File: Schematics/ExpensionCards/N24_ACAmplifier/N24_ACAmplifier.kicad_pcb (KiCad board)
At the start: 2 copper layers, 97 x 76 mm, 14 parts

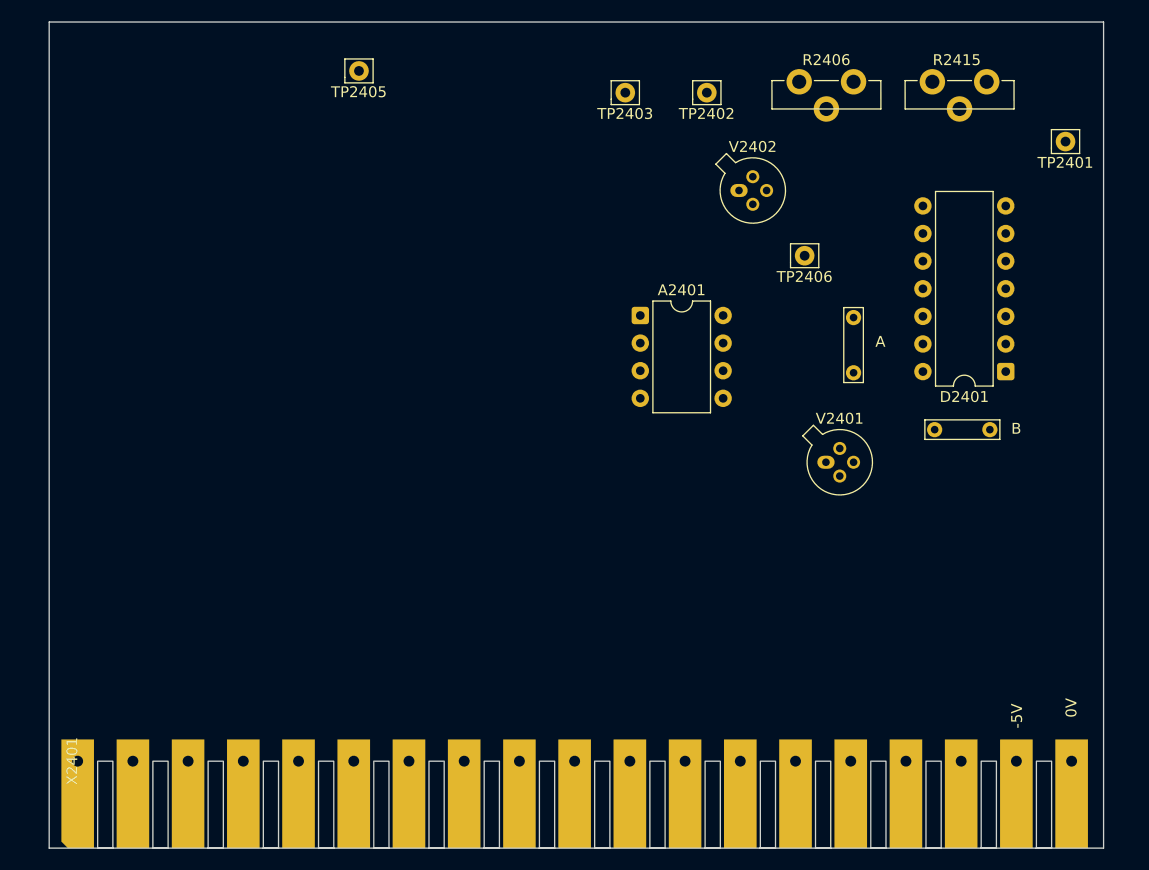
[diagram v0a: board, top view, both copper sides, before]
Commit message: Updated N24 schema/PCB
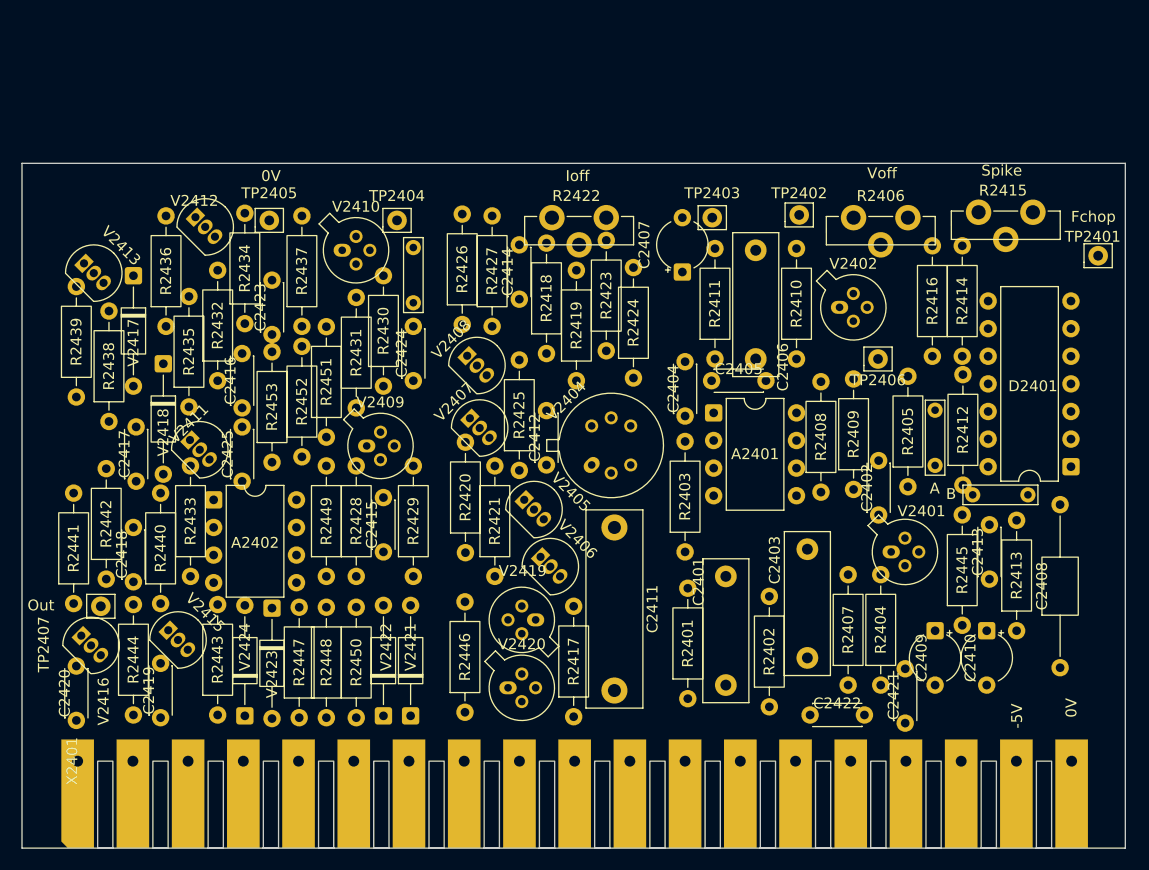
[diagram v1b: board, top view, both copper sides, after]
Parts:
- added A2402: LM393N, Package_DIP:DIP-8_W7.62mm, F.Cu at (114.1, 122.5)
- added C2401: 22n, Capacitor_THT:C_Rect_L13.0mm_W4.0mm_P10.00mm_FKS3_FKP3_MKS4, F.Cu at (161.2, 139.5)
- added C2402: 8p2, Capacitor_THT:C_Disc_D4.3mm_W1.9mm_P5.00mm, F.Cu at (175.3, 123.8)
- added C2403: 33n, Capacitor_THT:C_Rect_L13.0mm_W4.0mm_P10.00mm_FKS3_FKP3_MKS4, F.Cu at (168.8, 137.0)
- added C2404: 220p, Capacitor_THT:C_Disc_D4.3mm_W1.9mm_P5.00mm, F.Cu at (157.5, 114.8)
- added C2405: 3p9, Capacitor_THT:C_Disc_D4.3mm_W1.9mm_P5.00mm, F.Cu at (159.9, 111.5)
- added C2406: 220n, Capacitor_THT:C_Rect_L13.0mm_W4.0mm_P10.00mm_FKS3_FKP3_MKS4, F.Cu at (164.0, 109.5)
- added C2407: 22u, Capacitor_THT:CP_Radial_Tantal_D4.5mm_P5.00mm, F.Cu at (157.2, 101.5)
- added C2408: 13n3, Capacitor_THT:C_Axial_L5.1mm_D3.1mm_P15.00mm_Horizontal, F.Cu at (192.0, 137.9)
- added C2409: 6u8, Capacitor_THT:CP_Radial_Tantal_D4.5mm_P5.00mm, F.Cu at (180.5, 134.5)
- added C2410: 6u8, Capacitor_THT:CP_Radial_Tantal_D4.5mm_P5.00mm, F.Cu at (185.2, 134.5)
- added C2411: 330n, Capacitor_THT:C_Rect_L18.0mm_W5.0mm_P15.00mm_FKS3_FKP3, F.Cu at (151.0, 125.0)
- added C2412: 150p, Capacitor_THT:C_Disc_D4.3mm_W1.9mm_P5.00mm, F.Cu at (144.8, 119.2)
- added C2413: 10n, Capacitor_THT:C_Disc_D4.3mm_W1.9mm_P5.00mm, F.Cu at (185.5, 129.8)
- added C2414: 1n8, Capacitor_THT:C_Disc_D4.3mm_W1.9mm_P5.00mm, F.Cu at (142.2, 104.0)
- added C2415: 15p, Capacitor_THT:C_Disc_D4.3mm_W1.9mm_P5.00mm, F.Cu at (129.8, 127.2)
- added C2416: 12p, Capacitor_THT:C_Disc_D4.3mm_W1.9mm_P5.00mm, F.Cu at (116.8, 114.0)
- added C2417: 10n, Capacitor_THT:C_Disc_D4.3mm_W1.9mm_P5.00mm, F.Cu at (107.0, 120.8)
- added C2418: 560p, Capacitor_THT:C_Disc_D4.3mm_W1.9mm_P5.00mm, F.Cu at (106.8, 130.0)
- added C2419: 6n8, Capacitor_THT:C_Disc_D4.3mm_W1.9mm_P5.00mm, F.Cu at (109.2, 142.5)
- added C2420: 6n8, Capacitor_THT:C_Disc_D4.3mm_W1.9mm_P5.00mm, F.Cu at (101.5, 142.8)
- added C2421: 22n, Capacitor_THT:C_Disc_D4.3mm_W1.9mm_P5.00mm, F.Cu at (177.8, 143.0)
- added C2422: 22n, Capacitor_THT:C_Disc_D4.3mm_W1.9mm_P5.00mm, F.Cu at (169.0, 142.2)
- added C2423: 22n, Capacitor_THT:C_Disc_D4.3mm_W1.9mm_P5.00mm, F.Cu at (119.5, 107.2)
- added C2424: 22n, Capacitor_THT:C_Disc_D4.3mm_W1.9mm_P5.00mm, F.Cu at (132.5, 111.5)
- added C2425: 39p, Capacitor_THT:C_Disc_D4.3mm_W1.9mm_P5.00mm, F.Cu at (116.8, 120.8)
- added JP1: Jumper_2_Small_Bridged, TestPoint:TestPoint_Bridge_Pitch5.08mm_Drill0.7mm, F.Cu at (132.5, 104.3)
- added R2401: 1M00, Resistor_THT:R_Axial_DIN0207_L6.3mm_D2.5mm_P10.16mm_Horizontal, F.Cu at (157.8, 140.8)
- added R2402: 95k3, Resistor_THT:R_Axial_DIN0207_L6.3mm_D2.5mm_P10.16mm_Horizontal, F.Cu at (165.2, 141.5)
- added R2403: 9k53, Resistor_THT:R_Axial_DIN0207_L6.3mm_D2.5mm_P10.16mm_Horizontal, F.Cu at (157.5, 127.2)
- added R2404: 15E4, Resistor_THT:R_Axial_DIN0207_L6.3mm_D2.5mm_P10.16mm_Horizontal, F.Cu at (175.5, 139.5)
- added R2405: 681k, Resistor_THT:R_Axial_DIN0207_L6.3mm_D2.5mm_P10.16mm_Horizontal, F.Cu at (178.0, 121.2)
- added R2407: 1M00, Resistor_THT:R_Axial_DIN0207_L6.3mm_D2.5mm_P10.16mm_Horizontal, F.Cu at (172.5, 139.5)
- added R2408: 681k, Resistor_THT:R_Axial_DIN0207_L6.3mm_D2.5mm_P10.16mm_Horizontal, F.Cu at (170.0, 121.8)
- added R2409: 2k74, Resistor_THT:R_Axial_DIN0207_L6.3mm_D2.5mm_P10.16mm_Horizontal, F.Cu at (173.0, 121.5)
- added R2410: 15k4, Resistor_THT:R_Axial_DIN0207_L6.3mm_D2.5mm_P10.16mm_Horizontal, F.Cu at (167.8, 109.5)
- added R2411: 1M00, Resistor_THT:R_Axial_DIN0207_L6.3mm_D2.5mm_P10.16mm_Horizontal, F.Cu at (160.2, 109.5)
- added R2412: 1k05, Resistor_THT:R_Axial_DIN0207_L6.3mm_D2.5mm_P10.16mm_Horizontal, F.Cu at (183.1, 121.1)
- added R2413: 634k, Resistor_THT:R_Axial_DIN0207_L6.3mm_D2.5mm_P10.16mm_Horizontal, F.Cu at (188.0, 134.5)
- added R2414: 17k8, Resistor_THT:R_Axial_DIN0207_L6.3mm_D2.5mm_P10.16mm_Horizontal, F.Cu at (183.0, 109.2)
- added R2416: 1k21, Resistor_THT:R_Axial_DIN0207_L6.3mm_D2.5mm_P10.16mm_Horizontal, F.Cu at (180.2, 109.2)
- added R2417: 10M, Resistor_THT:R_Axial_DIN0207_L6.3mm_D2.5mm_P10.16mm_Horizontal, F.Cu at (147.2, 142.4)
- added R2418: 46k4, Resistor_THT:R_Axial_DIN0207_L6.3mm_D2.5mm_P10.16mm_Horizontal, F.Cu at (144.8, 109.0)
- added R2419: 46k4, Resistor_THT:R_Axial_DIN0207_L6.3mm_D2.5mm_P10.16mm_Horizontal, F.Cu at (147.5, 111.5)
- added R2420: 8k25, Resistor_THT:R_Axial_DIN0207_L6.3mm_D2.5mm_P10.16mm_Horizontal, F.Cu at (137.3, 127.3)
- added R2421: 8k25, Resistor_THT:R_Axial_DIN0207_L6.3mm_D2.5mm_P10.16mm_Horizontal, F.Cu at (140.0, 129.5)
- added R2422: 150, PM2528:Trimmer vertical, F.Cu at (150.2, 96.5)
- added R2423: 46k4, Resistor_THT:R_Axial_DIN0207_L6.3mm_D2.5mm_P10.16mm_Horizontal, F.Cu at (150.2, 108.8)
- added R2424: 10k, Resistor_THT:R_Axial_DIN0207_L6.3mm_D2.5mm_P10.16mm_Horizontal, F.Cu at (152.8, 111.2)
- added R2425: 2k74, Resistor_THT:R_Axial_DIN0207_L6.3mm_D2.5mm_P10.16mm_Horizontal, F.Cu at (142.2, 119.8)
- added R2426: 1k78, Resistor_THT:R_Axial_DIN0207_L6.3mm_D2.5mm_P10.16mm_Horizontal, F.Cu at (137.0, 106.3)
- added R2427: 140, Resistor_THT:R_Axial_DIN0207_L6.3mm_D2.5mm_P10.16mm_Horizontal, F.Cu at (139.8, 106.5)
- added R2428: 10M, Resistor_THT:R_Axial_DIN0207_L6.3mm_D2.5mm_P10.16mm_Horizontal, F.Cu at (127.2, 129.5)
- added R2429: 301k, Resistor_THT:R_Axial_DIN0207_L6.3mm_D2.5mm_P10.16mm_Horizontal, F.Cu at (132.5, 129.5)
- added R2430: 60k4, Resistor_THT:R_Axial_DIN0207_L6.3mm_D2.5mm_P10.16mm_Horizontal, F.Cu at (129.8, 112.0)
- added R2431: 2k15, Resistor_THT:R_Axial_DIN0207_L6.3mm_D2.5mm_P10.16mm_Horizontal, F.Cu at (127.2, 114.0)
- added R2432: 205, Resistor_THT:R_Axial_DIN0207_L6.3mm_D2.5mm_P10.16mm_Horizontal, F.Cu at (114.5, 111.5)
- added R2433: 2k61, Resistor_THT:R_Axial_DIN0207_L6.3mm_D2.5mm_P10.16mm_Horizontal, F.Cu at (112.0, 129.5)
- added R2434: 2k37, Resistor_THT:R_Axial_DIN0207_L6.3mm_D2.5mm_P10.16mm_Horizontal, F.Cu at (117.0, 106.2)
- added R2435: 7R05, Resistor_THT:R_Axial_DIN0207_L6.3mm_D2.5mm_P10.16mm_Horizontal, F.Cu at (111.9, 113.9)
- added R2436: 7R05, Resistor_THT:R_Axial_DIN0207_L6.3mm_D2.5mm_P10.16mm_Horizontal, F.Cu at (109.8, 106.5)
- added R2437: 2k15, Resistor_THT:R_Axial_DIN0207_L6.3mm_D2.5mm_P10.16mm_Horizontal, F.Cu at (122.2, 106.5)
- added R2438: 4k64, Resistor_THT:R_Axial_DIN0207_L6.3mm_D2.5mm_P10.16mm_Horizontal, F.Cu at (104.5, 115.2)
- added R2439: 215, Resistor_THT:R_Axial_DIN0207_L6.3mm_D2.5mm_P10.16mm_Horizontal, F.Cu at (101.5, 113.0)
- added R2440: 71R5, Resistor_THT:R_Axial_DIN0207_L6.3mm_D2.5mm_P10.16mm_Horizontal, F.Cu at (109.2, 132.0)
- added R2441: 71R5, Resistor_THT:R_Axial_DIN0207_L6.3mm_D2.5mm_P10.16mm_Horizontal, F.Cu at (101.2, 132.0)
- added R2442: 21R15, Resistor_THT:R_Axial_DIN0207_L6.3mm_D2.5mm_P10.16mm_Horizontal, F.Cu at (104.2, 129.8)
- added R2443: 71R5, Resistor_THT:R_Axial_DIN0207_L6.3mm_D2.5mm_P10.16mm_Horizontal, F.Cu at (114.5, 142.2)
- added R2444: 71R5, Resistor_THT:R_Axial_DIN0207_L6.3mm_D2.5mm_P10.16mm_Horizontal, F.Cu at (106.8, 142.2)
- added R2445: 1k05, Resistor_THT:R_Axial_DIN0207_L6.3mm_D2.5mm_P10.16mm_Horizontal, F.Cu at (183.0, 134.0)
- added R2446: 1k21, Resistor_THT:R_Axial_DIN0207_L6.3mm_D2.5mm_P10.16mm_Horizontal, F.Cu at (137.2, 142.0)
- added R2447: 15k4, Resistor_THT:R_Axial_DIN0207_L6.3mm_D2.5mm_P10.16mm_Horizontal, F.Cu at (122.0, 142.5)
- added R2448: 15k4, Resistor_THT:R_Axial_DIN0207_L6.3mm_D2.5mm_P10.16mm_Horizontal, F.Cu at (124.5, 142.5)
- added R2449: 46k4, Resistor_THT:R_Axial_DIN0207_L6.3mm_D2.5mm_P10.16mm_Horizontal, F.Cu at (124.5, 129.5)
- added R2450: 30k1, Resistor_THT:R_Axial_DIN0207_L6.3mm_D2.5mm_P10.16mm_Horizontal, F.Cu at (127.2, 142.5)
- added R2451: 1k05, Resistor_THT:R_Axial_DIN0207_L6.3mm_D2.5mm_P10.16mm_Horizontal, F.Cu at (124.5, 116.7)
- added R2452: 1k05, Resistor_THT:R_Axial_DIN0207_L6.3mm_D2.5mm_P10.16mm_Horizontal, F.Cu at (122.2, 118.5)
- added R2453: 30k1, Resistor_THT:R_Axial_DIN0207_L6.3mm_D2.5mm_P10.16mm_Horizontal, F.Cu at (119.5, 119.0)
- added TP2404: something, Connector_Pin:Pin_D0.9mm_L10.0mm_W2.4mm_FlatFork, F.Cu at (131.0, 96.8)
- added TP2407: OUT, Connector_Pin:Pin_D0.9mm_L10.0mm_W2.4mm_FlatFork, F.Cu at (103.8, 132.2)
- added V2404: BFQ14, Package_TO_SOT_THT:TO-75-6, F.Cu at (148.9, 119.2)
- added V2405: BC547B, Package_TO_SOT_THT:TO-92_Inline, F.Cu at (142.7, 122.5)
- added V2406: BC547B, Package_TO_SOT_THT:TO-92_Inline, F.Cu at (144.2, 127.7)
- added V2407: BC557B, Package_TO_SOT_THT:TO-92_Inline, F.Cu at (137.7, 115.0)
- added V2408: BC557B, Package_TO_SOT_THT:TO-92_Inline, F.Cu at (137.5, 109.2)
- added V2409: BFW11, Package_TO_SOT_THT:TO-72-4, F.Cu at (128.2, 117.5)
- added V2410: BFW11, Package_TO_SOT_THT:TO-72-4, F.Cu at (126.0, 99.5)
- added V2411: BF199, Package_TO_SOT_THT:TO-92_Inline, F.Cu at (112.0, 117.0)
- added V2412: BF199, Package_TO_SOT_THT:TO-92_Inline, F.Cu at (112.5, 96.5)
- added V2413: BC547B, Package_TO_SOT_THT:TO-92_Inline, F.Cu at (102.2, 100.7)
- added V2415: BF199, Package_TO_SOT_THT:TO-92_Inline, F.Cu at (110.0, 134.5)
- added V2416: BF324, Package_TO_SOT_THT:TO-92_Inline, F.Cu at (102.0, 135.0)
- added V2417: BZX79-C3V0, Diode_THT:D_DO-35_SOD27_P10.16mm_Horizontal, F.Cu at (106.8, 101.8)
- added V2418: BZV46-C2V0, Diode_THT:D_DO-35_SOD27_P10.16mm_Horizontal, F.Cu at (109.5, 109.9)
- added V2419: BAV45, Package_TO_SOT_THT:TO-72-4, F.Cu at (143.8, 133.5)
- added V2420: BAV45, Package_TO_SOT_THT:TO-72-4, F.Cu at (141.2, 139.8)
- added V2421: BAW62, Diode_THT:D_DO-35_SOD27_P10.16mm_Horizontal, F.Cu at (132.2, 142.3)
- added V2422: BAW62, Diode_THT:D_DO-35_SOD27_P10.16mm_Horizontal, F.Cu at (129.8, 142.3)
- added V2423: BZX79-B8V2, Diode_THT:D_DO-35_SOD27_P10.16mm_Horizontal, F.Cu at (119.5, 132.4)
- added V2424: BZX79-B8V2, Diode_THT:D_DO-35_SOD27_P10.16mm_Horizontal, F.Cu at (117.0, 142.3)
- moved TP2405 16.0 mm to (119.2, 96.8)
- moved V2402 14.2 mm to (171.7, 104.8)
- moved TP2402 14.1 mm to (168.0, 96.2)
- moved TP2403 14.0 mm to (160.0, 96.5)
- moved R2406 13.5 mm to (178.0, 96.5)
- moved R2415 12.7 mm to (189.5, 96.0)
- moved TP2406 11.7 mm to (175.2, 109.5)
- moved JP2401 11.4 mm to (180.5, 119.3)
- moved A2401 11.2 mm to (160.1, 114.5)
- moved TP2401 10.9 mm to (195.5, 100.0)
- moved D2401 10.6 mm to (193.0, 119.4)
- moved V2401 10.2 mm to (176.5, 127.2)
- moved JP2402 6.95 mm to (184.0, 122.0)
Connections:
- TP2402 pad 1: Net-(V2402-S) -> Net-(V2402-D)
- V2402 pad 2: Net-(V2402-S) -> GND4
- V2402 pad 3: GND4 -> Net-(V2402-D)
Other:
- board size 97 x 76 mm -> 101.5 x 63 mm
- board text added: "0V"
- board text added: "Fchop"
- board text added: "Ioff"
- board text added: "Out"
- board text added: "Spike"
- board text added: "Voff"
